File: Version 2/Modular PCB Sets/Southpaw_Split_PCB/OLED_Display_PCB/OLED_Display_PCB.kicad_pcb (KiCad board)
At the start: 2 copper layers, 77 x 46 mm, 3 parts, among them J3 Conn_01x07_Socket

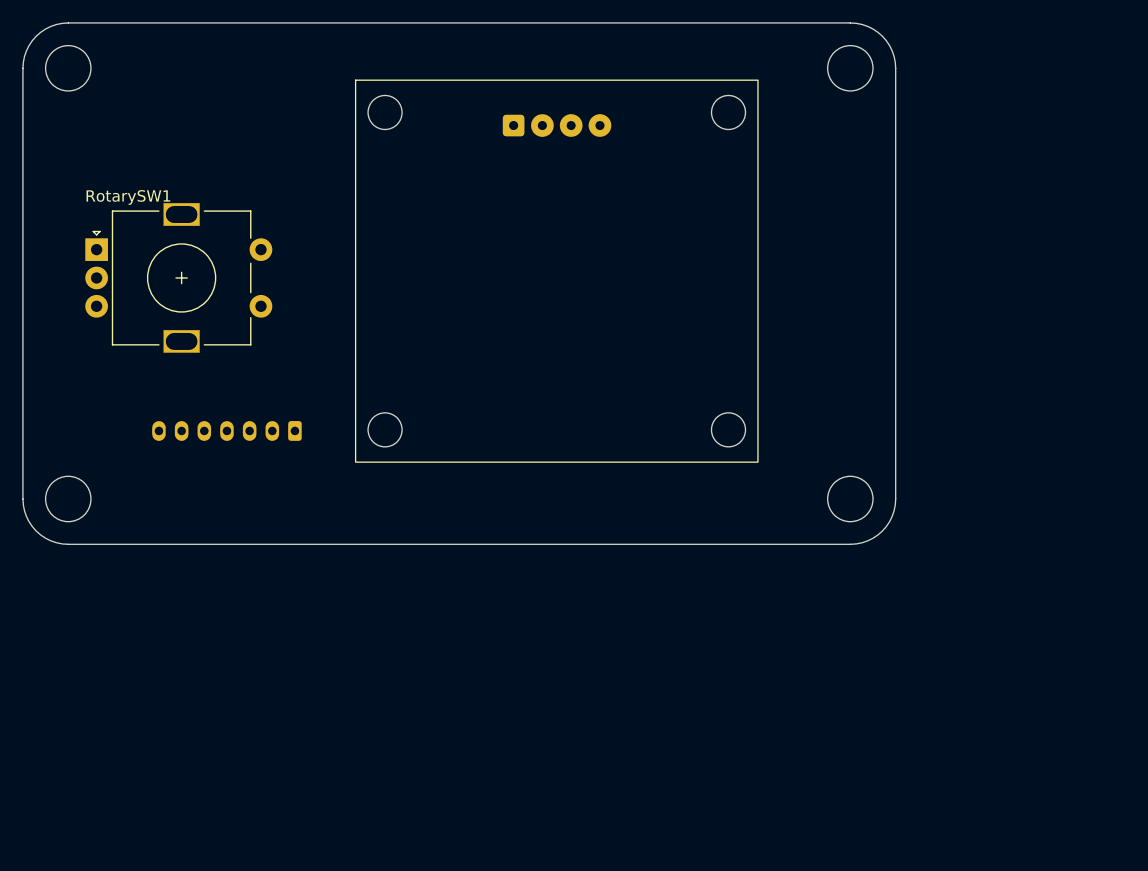
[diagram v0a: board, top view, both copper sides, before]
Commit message: Finalized design and uploaded gerbers to JLCpcb, waiting for boards to come in
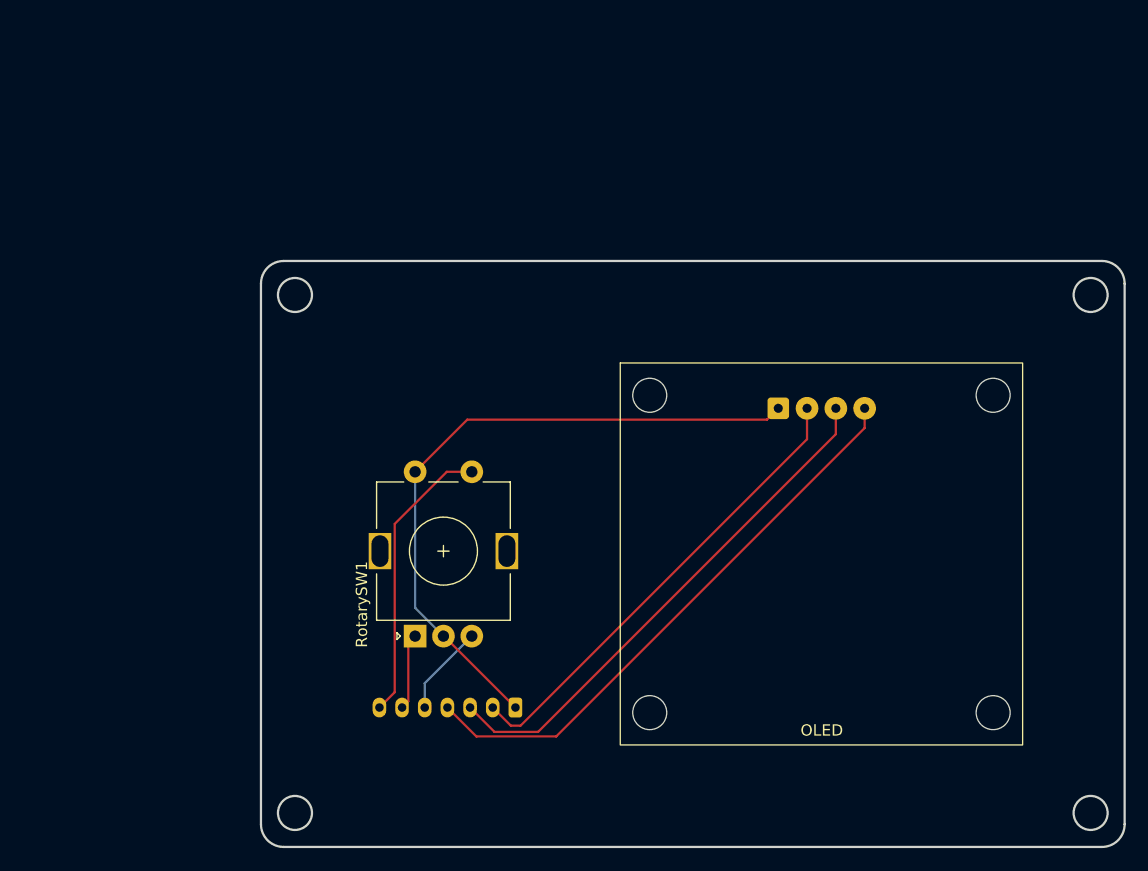
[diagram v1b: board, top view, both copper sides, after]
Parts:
- moved RotarySW1 44.2 mm to (105.6, 105.1), turned to 90 degrees
- moved OLED1 34.2 mm to (123.7, 114.7)
- moved J3 31.2 mm to (114.5, 111.4)
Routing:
- net /Gnd: track 0.00 -> 58.9 mm
- net /SDA: track 0.00 -> 50.9 mm
- net /SCK: track 0.00 -> 46.3 mm
- net /3V3: track 0.00 -> 41.6 mm
- net /Encoder_Press: track 0.00 -> 25.5 mm
- net /Rotary_Encoder_DT: track 0.00 -> 8.02 mm
- net /Rotary_Encoder_CLK: track 0.00 -> 6.78 mm
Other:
- board size 77 x 46 mm -> 76.2 x 51.7 mm
